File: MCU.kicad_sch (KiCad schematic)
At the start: 29 parts, among them J201 U.FL-R-SMT-1, SW201 TSA016, U201 ESP32-C3, U202 ZD25WQ32C, U203 WS2816C-1313, Y201 2.D.1.400000920 40MHz

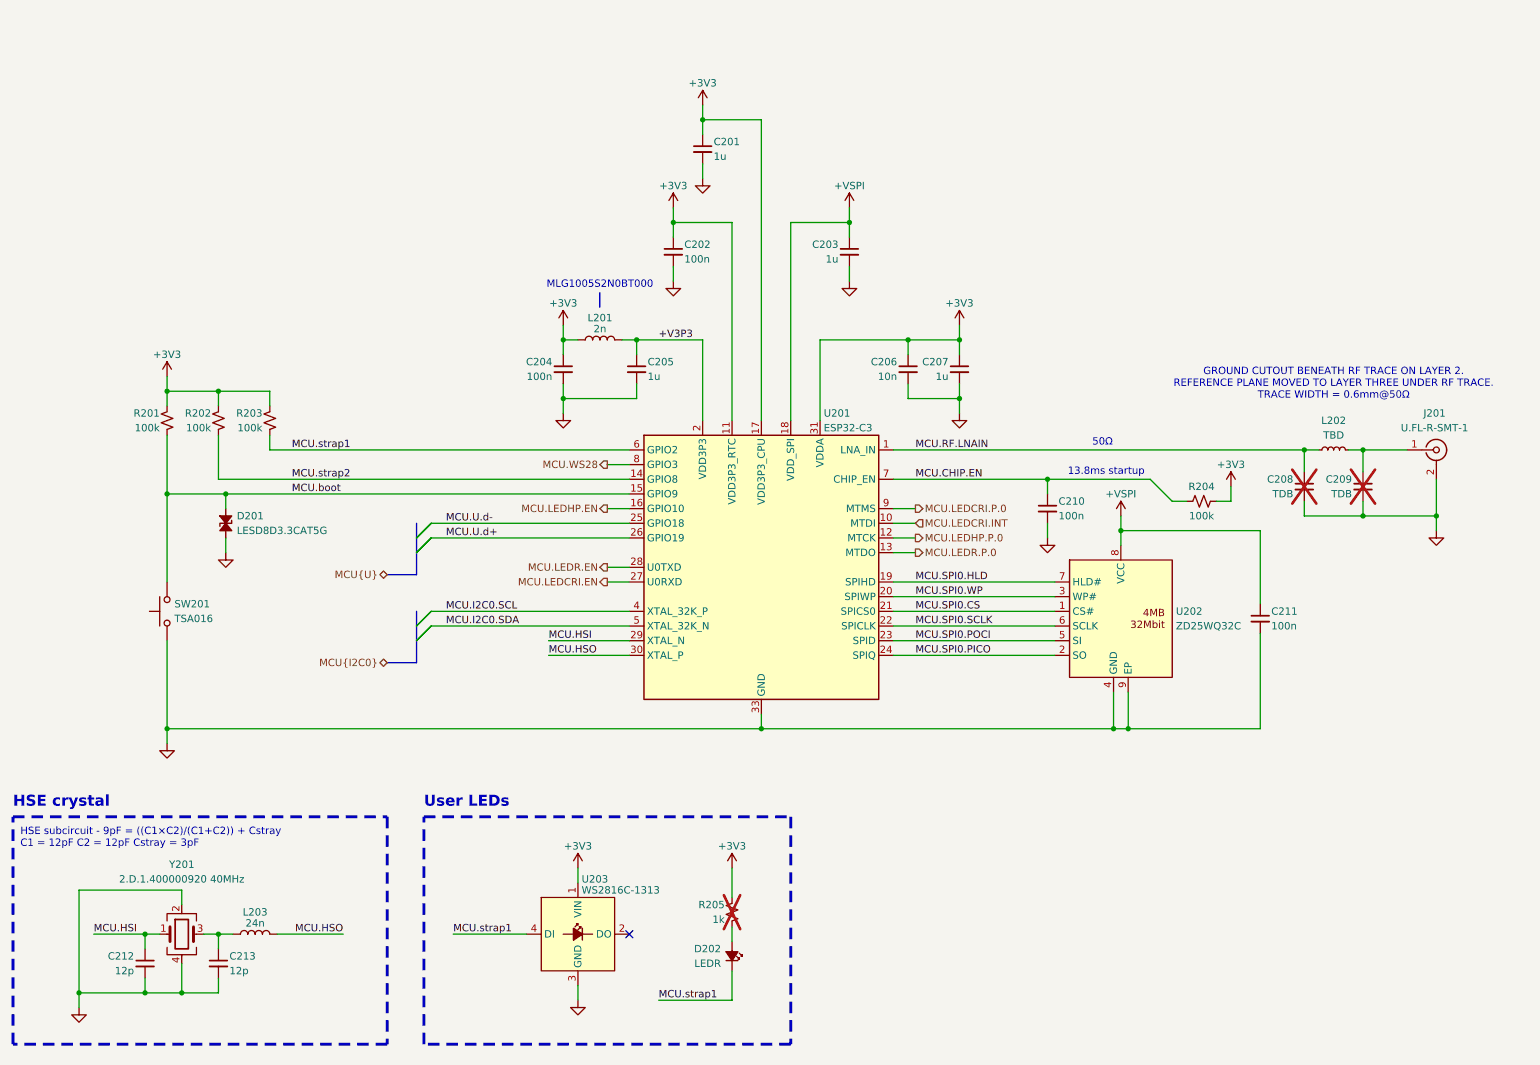
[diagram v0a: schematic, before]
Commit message: Add files via upload
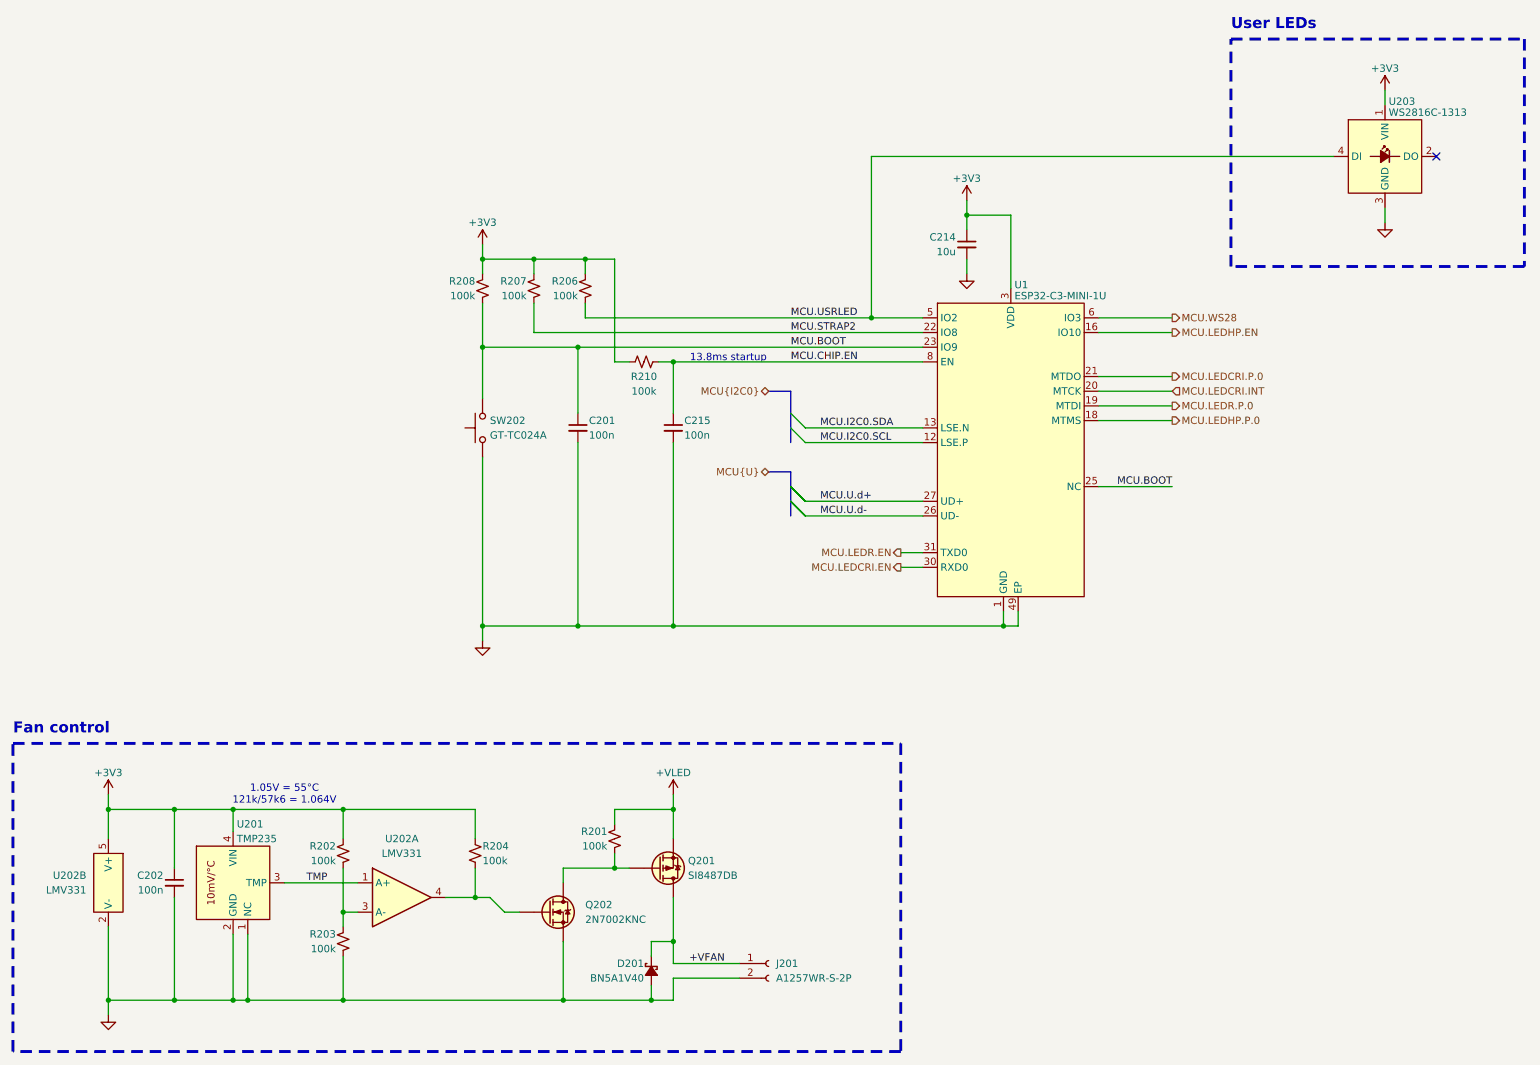
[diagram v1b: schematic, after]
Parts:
- removed C203, C205, C207: 1u, Perfect passives:C 0402 (1005 Metric), symbol Device:C_Small
- removed C204, C210, C211: 100n, Perfect passives:C 0402 (1005 Metric), symbol Device:C_Small
- removed C206: 10n, Perfect passives:C 0402 (1005 Metric), symbol Device:C_Small
- removed C208, C209: TDB, Perfect passives:C 0402 (1005 Metric), symbol Device:C_Small
- removed C212, C213: 12p, Perfect passives:C 0402 (1005 Metric), symbol Device:C_Small
- removed D201: LESD8D3.3CAT5G, DFN-x:DFN-1006-2L, symbol TVS diodes bidirectional:LESD8D3.3CAT5G
- removed D202: LEDR, LED SMD:LED-0402-R, symbol SMD LED:NCD0402R1
- removed J201: U.FL-R-SMT-1, RF connectors:U.FL-R-1, symbol Connector:Conn_Coaxial
- removed L201: 2n, Perfect passives:L 0402 (1005 Metric), symbol Device:L
- removed L202: TBD, Perfect passives:L 0402 (1005 Metric), symbol Device:L_Small
- removed L203: 24n, Perfect passives:L 0402 (1005 Metric), symbol Device:L
- removed R205: 1k, Perfect passives:R 0402 (1005 Metric), symbol Device:R_Small_US
- removed SW201: TSA016, Buttons SMD:TSA016, symbol Switch:SW_Push
- removed U201: ESP32-C3, QFN-x generic:QFN-32 (5x5) P0.5 ESP, symbol MCU_Espressif:ESP32-C3
- removed U202: ZD25WQ32C, SON-xx:USON-8 (2x3) P0.5, symbol NOR Flash:ZD25Q32C 4MB
- removed Y201: 2.D.1.400000920 40MHz, Crystals SMD:SMD-2016-4P, symbol Device:Crystal_GND24
- added C214: 10u, Perfect passives:C 0805 (2012 Metric), symbol Device:C_Small
- added C215: 100n, Perfect passives:C 0402 (1005 Metric), symbol Device:C_Small
- added D201: BN5A1V40, DFN-x:DFN1610-2L (1.6x1), symbol Schottky diodes:BN5A1V40
- added J201: A1257WR-S-2P, Connectors SMD:A1257WR-S-2P (GH), symbol Connector:Conn_01x02_Socket
- added Q201: SI8487DB, CSP-xxx:WLCSP-4 (1.56x1.56) P0.8, symbol Mosfets P-channel:SI8487DB-T1-E1
- added Q202: 2N7002KNC, DFN-x:DFN-1006-3L, symbol Mosfet N-channel:2N7002KNC
- added R206, R207, R208, R210: 100k, Perfect passives:R 0402 (1005 Metric), symbol Device:R_Small_US
- added SW202: GT-TC024A, Buttons SMD:GT-TC024A-H0060-L1, symbol Switch:SW_Push
- added U1: ESP32-C3-MINI-1U, RF modules:ESP32-C3-MINI-1U, symbol Modules RF:ESP32-C3-MINI-1U
- added U201: TMP235, SOT-xxx:SOT-363-5, symbol Temperature sensors:TMP235A4DCK
- added U202: LMV331, SOT-xxx:SOT-363-5, symbol Comparators:LMV331DCK
- C201: value 1u -> 100n
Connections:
- net +3V3: now also C214.1, R206.2, R207.2, R208.2, R210.1, U1.3 (VDD), U201.4 (VIN), U202.5 (V+); no longer C201.1, R201.2, R203.2
- net GND: now also R203.1, C214.2, C215.2, D201.2 (A), J201.2 (Pin_2), Q202.2 (S), SW202.1, U1.1 (GND), U1.11 (GND), U1.14 (GND), U1.2 (GND), U1.36 (GND), U1.37 (GND), U1.38 (GND), U1.39 (GND), U1.40 (GND), U1.41 (GND), U1.42 (GND), U1.43 (GND), U1.44 (GND), U1.45 (GND), U1.46 (GND), U1.47 (GND), U1.48 (GND), U1.49 (EP), U1.50 (GND), U1.51 (GND), U1.52 (GND), U1.53 (GND), U201.1 (NC), U201.2 (GND), U201.5 (NC), U202.2 (V-)
- net MCU.CHIP.EN: now also C215.1, R210.2, U1.8 (EN); no longer R204.1
- net MCU.I2C0.SCL: now also U1.12 (LSE.P)
- net MCU.I2C0.SDA: now also U1.13 (LSE.N)
- net MCU.LEDCRI.EN: now also U1.30 (RXD0)
- net MCU.LEDCRI.INT: now also U1.20 (MTCK)
- net MCU.LEDCRI.P.0: now also U1.21 (MTDO)
- net MCU.LEDHP.EN: now also U1.16 (IO10)
- net MCU.LEDHP.P.0: now also U1.18 (MTMS)
- net MCU.LEDR.EN: now also U1.31 (TXD0)
- net MCU.LEDR.P.0: now also U1.19 (MTDI)
- net MCU.U.d+: now also U1.27 (UD+)
- net MCU.U.d-: now also U1.26 (UD-)
- net MCU.WS28: now also U1.6 (IO3)
- net MCU.boot: no longer names the net of R201.1
- net MCU.boot: now also Q201.1 (G), Q202.3 (D)
- net MCU.strap1 renamed MCU.USRLED
- net MCU.USRLED: now also R206.1, U1.5 (IO2); no longer R203.1
- net MCU.strap2: no longer names the net of R202.1
- net MCU.strap2: now also R203.2, U202.3 (A-)
- new net: Q202.1 (G), R204.1, U202.4
- new net: U1.10 (NC), U1.15 (NC), U1.17 (NC), U1.24 (NC), U1.28 (NC), U1.29 (NC), U1.32 (NC), U1.33 (NC), U1.34 (NC), U1.35 (NC), U1.4 (NC), U1.7 (NC), U1.9 (NC)
- new net +VFAN: D201.1 (K), J201.1 (Pin_1), Q201.2 (D), Q201.3 (D)
- new net +VLED: Q201.4 (S), R201.2
- new net MCU.BOOT: C201.1, R208.1, SW202.2, U1.23 (IO9), U1.25 (NC)
- new net MCU.STRAP2: R207.1, U1.22 (IO8)
- new net TMP: U201.3 (TMP), U202.1 (A+)
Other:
- note added: "1.05V = 55°C 121k/57k6 = 1.064V"
- note added: "Fan control"
- note removed: "50Ω"
- note removed: "GROUND CUTOUT BENEATH RF TRACE ON LAYER 2. REFERENCE PLANE MOVED TO LAYER THREE UNDER RF TRACE. TRACE WIDTH = 0.6mm@50Ω"
- note removed: "HSE crystal"
- note removed: "HSE subcircuit - 9pF = ((C1×C2)/(C1+C2)) + Cstray C1 = 12pF C2 = 12pF Cstray = 3pF"
- note removed: "MLG1005S2N0BT000"
- moved on the sheet: U203
